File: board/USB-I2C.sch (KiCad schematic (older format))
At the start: 17 parts, among them J1 USB_OTG, J2 Conn_01x06, U1 SPX3819, U2 STM32F042K4Tx, X1 I2C-6P, X2 I2C, X3 SWD

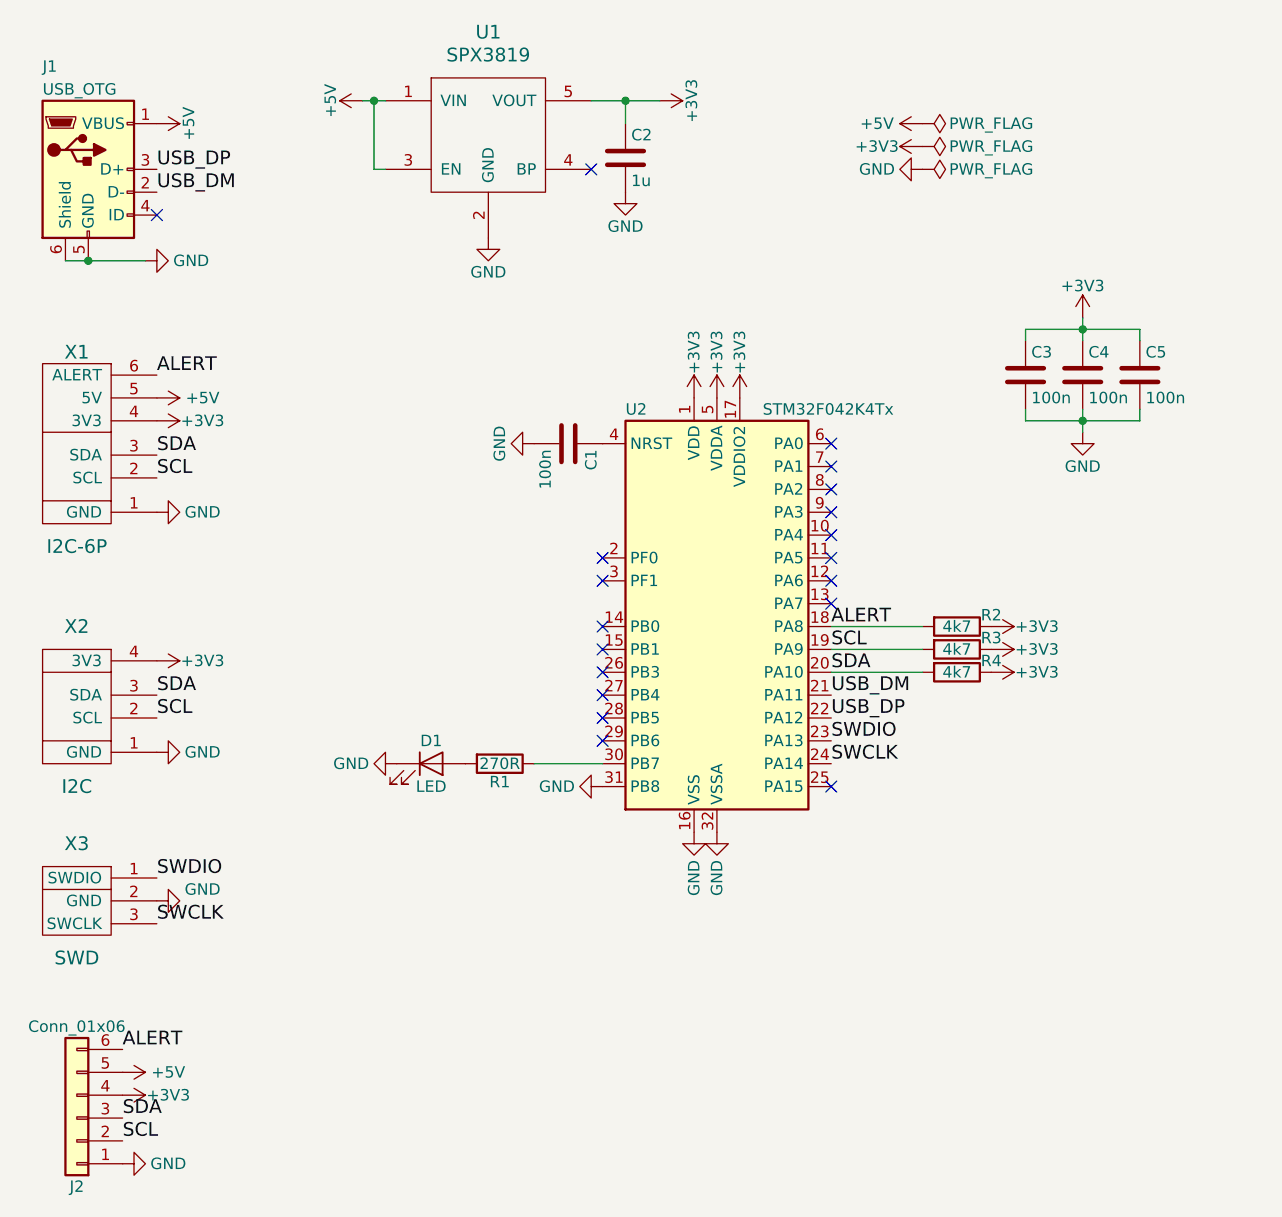
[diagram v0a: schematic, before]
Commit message: WIP
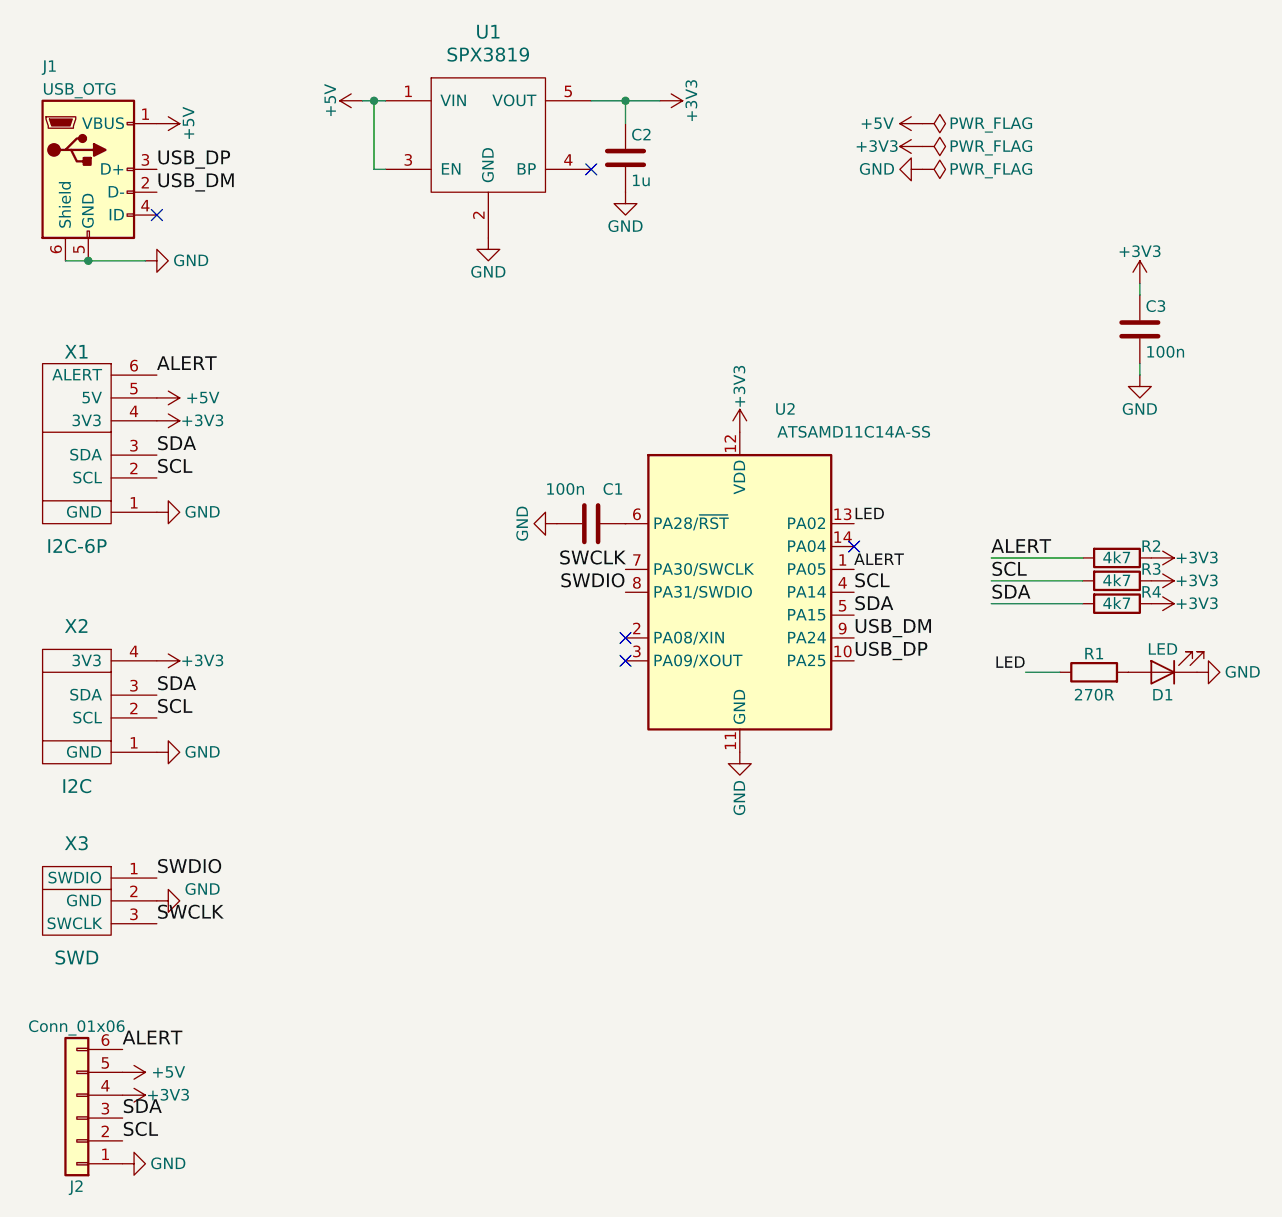
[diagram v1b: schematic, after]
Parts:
- removed C4, C5: 100n, Capacitor_SMD:C_0805_2012Metric, symbol Device:C
- removed U2: STM32F042K4Tx, Package_QFP:LQFP-32_7x7mm_P0.8mm, symbol MCU_ST_STM32F0:STM32F042K4Tx
- added U2: ATSAMD11C14A-SS, Package_SO:SOIC-14_3.9x8.7mm_P1.27mm, symbol MCU_Microchip_SAMD:ATSAMD11C14A-SS
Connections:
- net +3V3: now also U2.12 (VDD)
- net ALERT: now also U2.1 (PA05)
- net GND: now also U2.11 (GND)
- net SCL: now also U2.4 (PA14)
- net SDA: now also U2.5 (PA15)
- net SWCLK: now also U2.7 (PA30/SWCLK)
- net SWDIO: now also U2.8 (PA31/SWDIO)
- net USB_DM: now also U2.9 (PA24)
- net USB_DP: now also U2.10 (PA25)
- net LED: now reaches R1.1
- net LED: now also U2.13 (PA02)
- net at C1.1: now also U2.6 (PA28/~RST)
- no-connect marks 19 -> 5
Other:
- moved on the sheet: C1, C3, D1, R1, R2, R3, R4
